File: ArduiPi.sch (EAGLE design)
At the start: 96 parts, among them IC1 AVR-MEGA8-PPTH, IC2 DS2482-100S, J1 Teleinfo, J10 ICSP, J11 DNP, J12 DNP, J13 DNP, J14 DNP, J15 DNP, J16 DNP, J17 DNP, J18 DNP, J19 DNP, J2 DNP, J3 DNP, J4 DNP, J5 DNP, J6 DNP, J7 DNP, J8 DNP, J9 DC-044-AH, K1 RESET, Q1 BSS138, Q2 BSS138, Q3 BSS138, Q4 BSS138, Q5 BSS84, U1 78M05, U2 LD1117 3V3, U3 TXB0104, U4 TXB0108, U5 TXB0108, X1 16Mhz

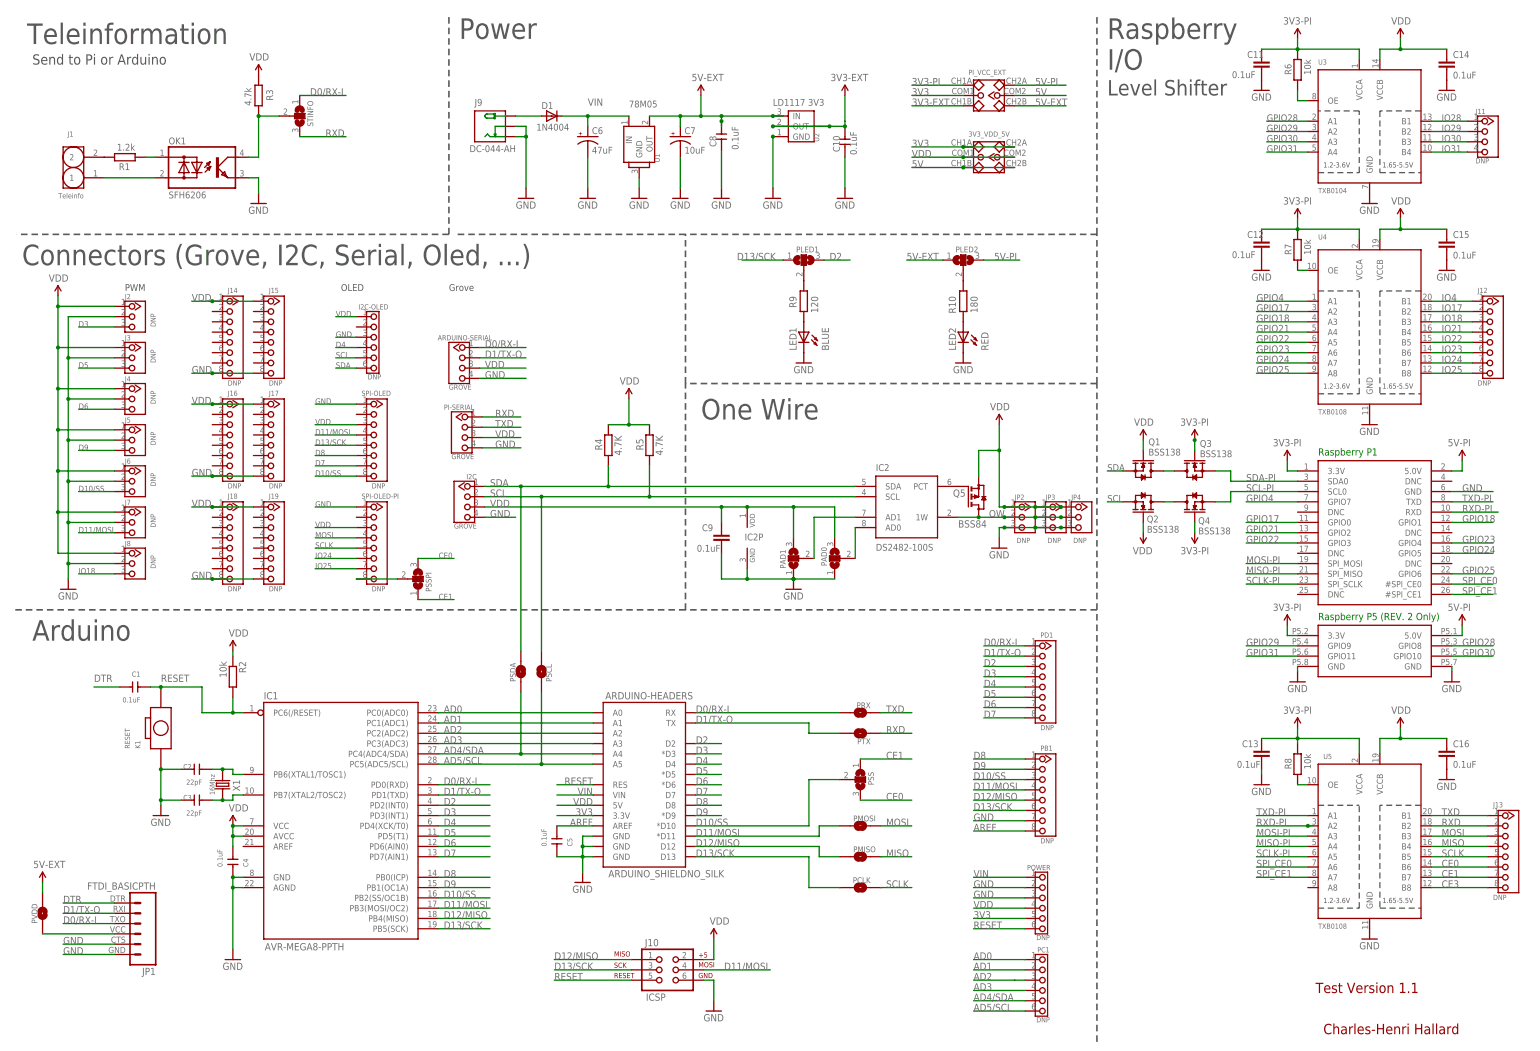
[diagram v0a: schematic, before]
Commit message: Prototype Board
ArduiPi First Prototype Board
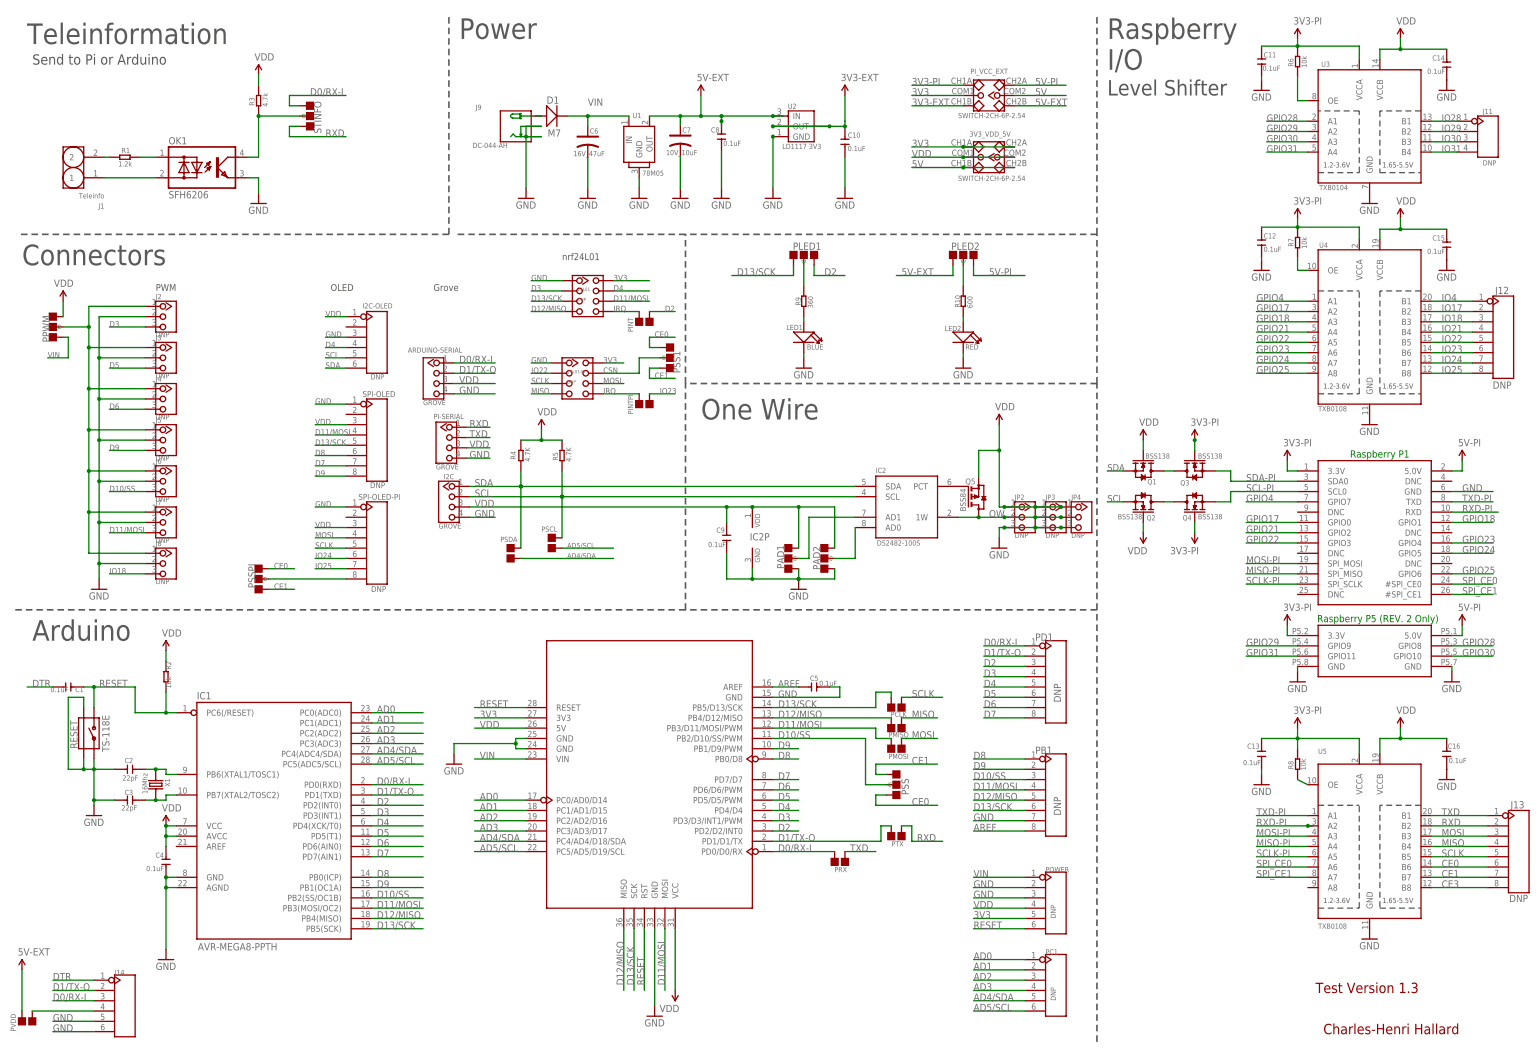
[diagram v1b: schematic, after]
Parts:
- removed ARDUINO-HEADERS: ARDUINO_SHIELDNO_SILK, SparkFun-Boards:ARDUINO_SHIELDNO_SILK
- removed J10: ICSP, SparkFun:AVR_SPI_PRG_6PTH
- removed J15, J16, J17, J18, J19: DNP, Seeedstudio-Connector:HEADER-8P-2.54
- removed JP1: FTDI_BASICPTH, SparkFun-Connectors:FTDI_BASICPTH
- removed K1: RESET, Seeedstudio-Discrete.rpt:BOTTON-2P-90
- added 24L01, 24L01-PI: DNP, Seeedstudio-Connector:HEADER-2X4P-2.54
- added PINT: PINT, Discrete:PAD-JUMPER-2P
- added PINTPI: PINTPI, Discrete:PAD-JUMPER-2P
- added PPWM, PSS1: (no value), Discrete:PAD-JUMPER-3P-40*40
- added RESET: TS-118E, Discrete:BUTTON-4P-REINFORCE'TS-118E'
- added U6: (no value), For_Test_Albert_v6:ARDUINO'W/-SILK
- C1, C10, C2, C3, C4, C5, C8: device Seeedstudio-Discrete.rpt:C'1.4' -> Discrete:C-0603
- C11, C12, C13, C14, C15, C16, C9: device resistor:C-EUC0603 -> Discrete:C-0603
- C6: value 47uF -> 16V_47uF; device SparkFun:CAP_POLPTH2 -> Discrete:CAP-AVX-C
- C7: value 10uF -> 10V_10uF; device SparkFun:CAP_POLPTH2 -> Discrete:CAP-AVX-A
- D1: value 1N4004 -> M7; device adafruit:1N4004 -> Discrete:D'SMA'
- I2C-OLED, PC1, POWER: device Seeedstudio-Connector:HEADER-6P-2.54 -> Connector:HEADER-6P-65/35MIL
- J11: device Seeedstudio-Connector:HEADER-4P-80/40MIL -> Connector:HEADER-4P-65/35MIL
- J12, J13, PB1, PD1, SPI-OLED, SPI-OLED-PI: device Seeedstudio-Connector:HEADER-8P-2.54 -> Connector:HEADER-8P-65/35MIL
- J14: value DNP -> (none); device Seeedstudio-Connector:HEADER-8P-2.54 -> Connector:HEADER-6P-65/35MIL
- J9: device For_Test_Albert:DC-044 -> Connector:JACK-DC-044
- LED1, LED2: device led:LEDCHIP-LED0603 -> Discrete:LED'0603'
- PAD1: value PAD1 -> (none); device Seeedstudio-Discreter.rpt:PAD-SOLDERJUMPER-2WAYS -> Discrete:PAD-JUMPER-3P-40*40; PARTNO (none) -> DNP
- PAD2: value PAD0 -> (none); device Seeedstudio-Discreter.rpt:PAD-SOLDERJUMPER-2WAYS -> Discrete:PAD-JUMPER-3P-40*40; PARTNO (none) -> DNP
- PCLK, PMISO, PMOSI, PRX, PSCL, PSDA, PTX, PVDD: device Seeedstudio-Discreter.rpt:PAD-SOLDERJUMPERNC -> Discrete:PAD-JUMPER-2P
- PLED1: value PLED1 -> (none); device Seeedstudio-Discreter.rpt:PAD-SOLDERJUMPER-2WAYS -> Discrete:PAD-JUMPER-3P-40*40; PARTNO (none) -> DNP
- PLED2: value PLED2 -> (none); device Seeedstudio-Discreter.rpt:PAD-SOLDERJUMPER-2WAYS -> Discrete:PAD-JUMPER-3P-40*40
- PSS: value PSS -> (none); device Seeedstudio-Discreter.rpt:PAD-SOLDERJUMPER-2WAYS -> Discrete:PAD-JUMPER-3P-40*40
- PSSPI: value PSSPI -> (none); device Seeedstudio-Discreter.rpt:PAD-SOLDERJUMPER-2WAYS -> Discrete:PAD-JUMPER-3P-40*40; PARTNO (none) -> DNP
- R1, R2, R3, R4, R5: device resistor:R-EU_R0805 -> Discrete:R-0603
- R10: value 180 -> 600; device resistor:R-EU_R0805 -> Discrete:R-0603
- R6, R7, R8: device resistor:R-EU_R0603 -> Discrete:R-0603
- R9: value 120 -> 360; device resistor:R-EU_R0805 -> Discrete:R-0603
- STINFO: value STINFO -> (none); device Seeedstudio-Discreter.rpt:PAD-SOLDERJUMPER-2WAYS -> Discrete:PAD-JUMPER-3P-40*40
- X1: device Seeedstudio-Discrete.rpt:CRYSTAL-HC49S -> Discrete:CRYSTAL'5032'
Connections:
- new net CSN: 24L01-PI.7, PSS1.C
- new net IRQ: 24L01-PI.5, 24L01.5, PINT.2, PINTPI.2
- new net N$21: J2.P$1, J3.P$1, J4.P$1, J5.P$1, J6.P$1, J7.P$1, J8.P$1, PPWM.C
- net 3V3: now also 24L01-PI.8, 24L01.8, U6.3V3; no longer ARDUINO-HEADERS.3.3V
- net 5V-EXT: now also PLED2.L; no longer PLED2.1
- net 5V-PI: now also PLED2.R; no longer PLED2.3
- net AD0: now also U6.PC0/AD0/D14; no longer ARDUINO-HEADERS.A0
- net AD1: now also U6.PC1/AD1/D15; no longer ARDUINO-HEADERS.A1
- net AD2: now also U6.PC2/AD2/D16; no longer ARDUINO-HEADERS.A2
- net AD3: now also U6.PC3/AD3/D17; no longer ARDUINO-HEADERS.A3
- net AD4/SDA: now also U6.PC4/AD4/D18/SDA; no longer ARDUINO-HEADERS.A4
- net AD5/SCL: now also U6.PC5/AD5/D19/SCL; no longer ARDUINO-HEADERS.A5
- net AREF: now also C5.1, U6.AREF; no longer ARDUINO-HEADERS.AREF, C5.2
- net CE0: now also PSS.R, PSS1.L, PSSPI.R; no longer PSS.3, PSSPI.3
- net CE1: now also PSS.L, PSS1.R, PSSPI.L; no longer PSS.1, PSSPI.1
- net D0/RX-I: now also J14.3, STINFO.L, U6.PD0/D0/RX; no longer ARDUINO-HEADERS.RX, JP1.3, STINFO.1
- net D1/TX-O: now also J14.2, U6.PD1/D1/TX; no longer ARDUINO-HEADERS.TX, JP1.2
- net D10/SS: now also PSS.C, U6.PB2/D10/SS/PWM; no longer ARDUINO-HEADERS.*D10, PSS.2, SPI-OLED.8
- net D11/MOSI: now also 24L01.6, U6.MOSI, U6.PB3/D11/MOSI/PWM; no longer ARDUINO-HEADERS.*D11, J10.4
- net D12/MISO: now also 24L01.4, U6.MISO, U6.PB4/D12/MISO; no longer ARDUINO-HEADERS.D12, J10.1
- net D13/SCK: now also 24L01.3, PLED1.L, U6.PB5/D13/SCK, U6.SCK; no longer ARDUINO-HEADERS.D13, J10.3, PLED1.1
- net D2: now also PINT.1, PLED1.R, U6.PD2/D2/INT0; no longer ARDUINO-HEADERS.D2, PLED1.3
- net D3: now also 24L01.2, U6.PD3/D3/INT1/PWM; no longer ARDUINO-HEADERS.*D3
- net D4: now also 24L01.7, U6.PD4/D4; no longer ARDUINO-HEADERS.D4
- net D5: now also U6.PD5/D5/PWM; no longer ARDUINO-HEADERS.*D5
- net D6: now also U6.PD6/D6/PWM; no longer ARDUINO-HEADERS.*D6
- net D7: now also U6.PD7/D7; no longer ARDUINO-HEADERS.D7
- net D8: now also U6.PB0/D8; no longer ARDUINO-HEADERS.D8
- net D9: now also SPI-OLED.8, U6.PB1/D9/PWM; no longer ARDUINO-HEADERS.*D9
- net DTR: now also J14.1; no longer JP1.1
- net GND: now also 24L01-PI.1, 24L01.1, C5.2, J14.5, J14.6, LED1.-, LED2.-, PAD1.L, PAD2.L, RESET.1, RESET.S1, RESET.S2, U6.GND, U6.GND@0, U6.GND@1, U6.GND@2; no longer ARDUINO-HEADERS.GND@0, ARDUINO-HEADERS.GND@1, ARDUINO-HEADERS.GND@2, C5.1, J10.6, J14.8, J15.8, J16.8, J17.8, J18.8, J19.8, JP1.5, JP1.6, K1.1, LED1.C, LED2.C, PAD1.1, PAD2.1
- net IO22: now also 24L01-PI.2
- net IO23: now also PINTPI.1
- net MISO: now also 24L01-PI.4
- net MOSI: now also 24L01-PI.6
- net N$1: now also STINFO.C; no longer STINFO.2
- net N$10: now also J14.4; no longer JP1.4
- net N$11: now also PAD1.C; no longer PAD1.2
- net N$12: now also D1.+; no longer D1.A
- net N$16: now also PLED1.C; no longer PLED1.2
- net N$17: now also LED1.+; no longer LED1.A
- net N$18: now also LED2.+; no longer LED2.A
- net N$2: now also PAD2.C; no longer PAD2.2
- net N$20: now also PLED2.C; no longer PLED2.2
- net RESET: now also RESET.2, U6.RESET, U6.RST; no longer ARDUINO-HEADERS.RES, J10.5, K1.2
- net RXD: now also STINFO.R; no longer STINFO.3
- net SCLK: now also 24L01-PI.3
- net SSPI: now also PSSPI.C; no longer PSSPI.2
- net VDD: now also PAD1.R, PAD2.R, PPWM.L, U6.5V, U6.VCC; no longer ARDUINO-HEADERS.5V, J10.2, J14.1, J15.1, J16.1, J17.1, J18.1, J19.1, J2.P$1, J3.P$1, J4.P$1, J5.P$1, J6.P$1, J7.P$1, J8.P$1, PAD1.3, PAD2.3
- net VIN: now also D1.-, PPWM.R, U6.VIN; no longer ARDUINO-HEADERS.VIN, D1.C
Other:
- note added: "Connectors"
- note added: "Test Version 1.3"
- note added: "nrf24L01"
- note removed: "Connectors (Grove, I2C, Serial, Oled, ...)"
- note removed: "Test Version 1.1"
- moved on the sheet: ARDUINO-SERIAL, C1, C2, C3, C4, C5, I2C, IC1, IC2P, J2, J3, J4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
